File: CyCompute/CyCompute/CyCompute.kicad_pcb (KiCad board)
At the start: 2 copper layers, 100 x 140 mm, 29 parts, among them J1 RJ45, J10 RJ11, J11 RJ11, J12 RJ11, J13 RJ11, J14 RJ45, J15 RJ11, J16 USB_A, J17 USB_A, J18 Conn_01x04_Female, J2 RJ45, J3 RJ45, J4 RJ45, J5 RJ45, J6 CAM0, J7 CAM1, J8 Pi Std header, J9 RJ11, U1 TCA9548APWR, U2 LAN9514, U3 P82B715DR, U4 IP4234CZ6, U5 IP4234CZ6, U6 PAM2306AYPKE, U7 SP2526A-2EN-L

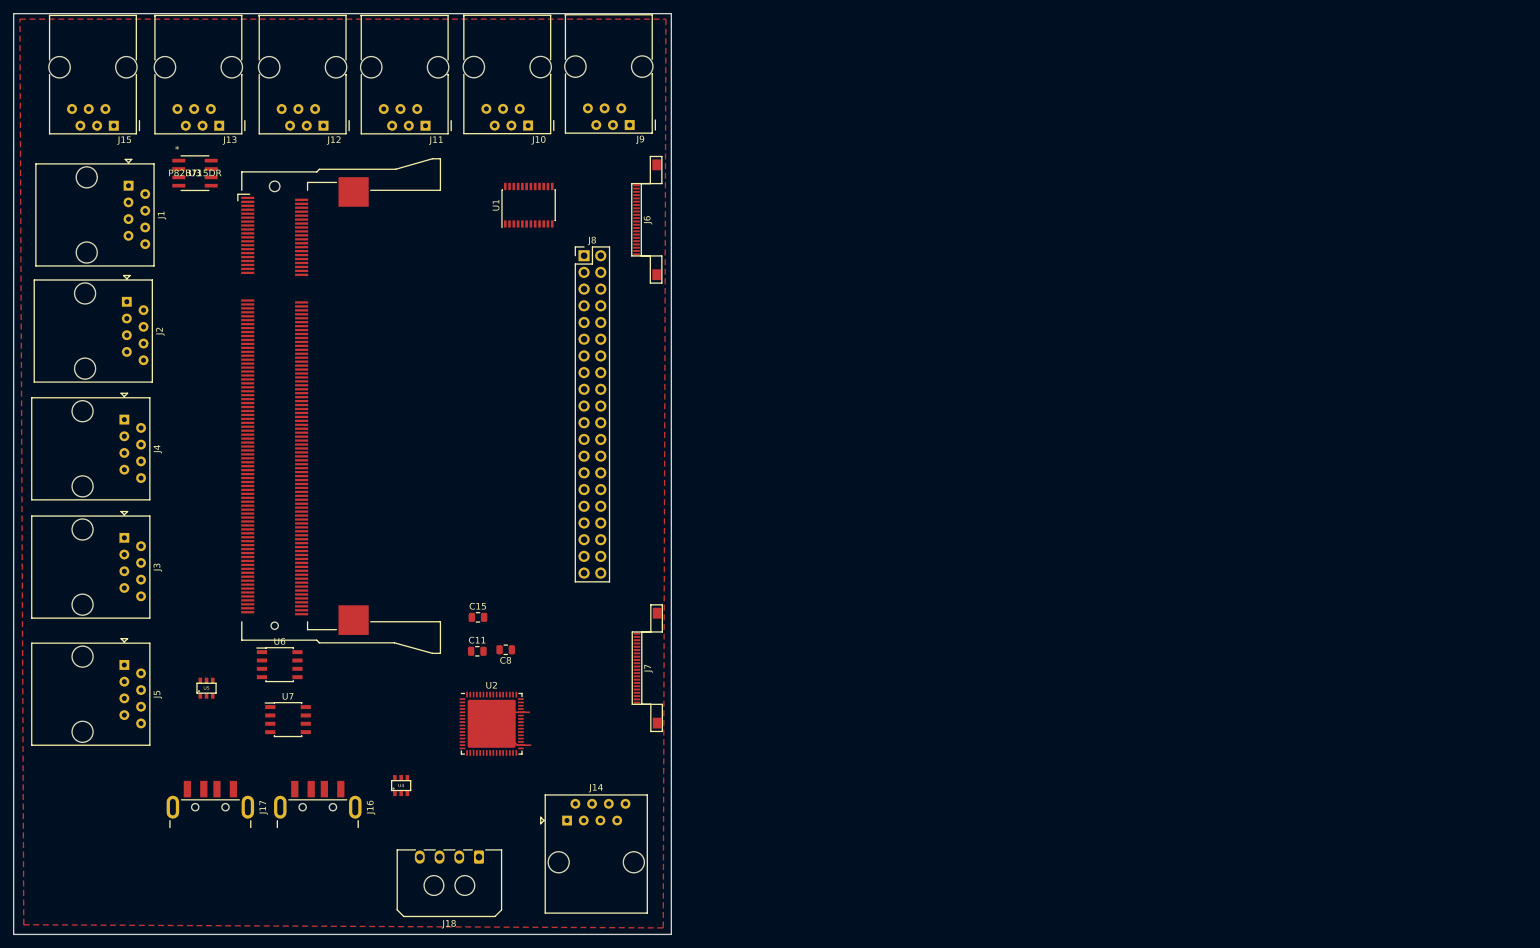
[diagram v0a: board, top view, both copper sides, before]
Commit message: Getting up to date
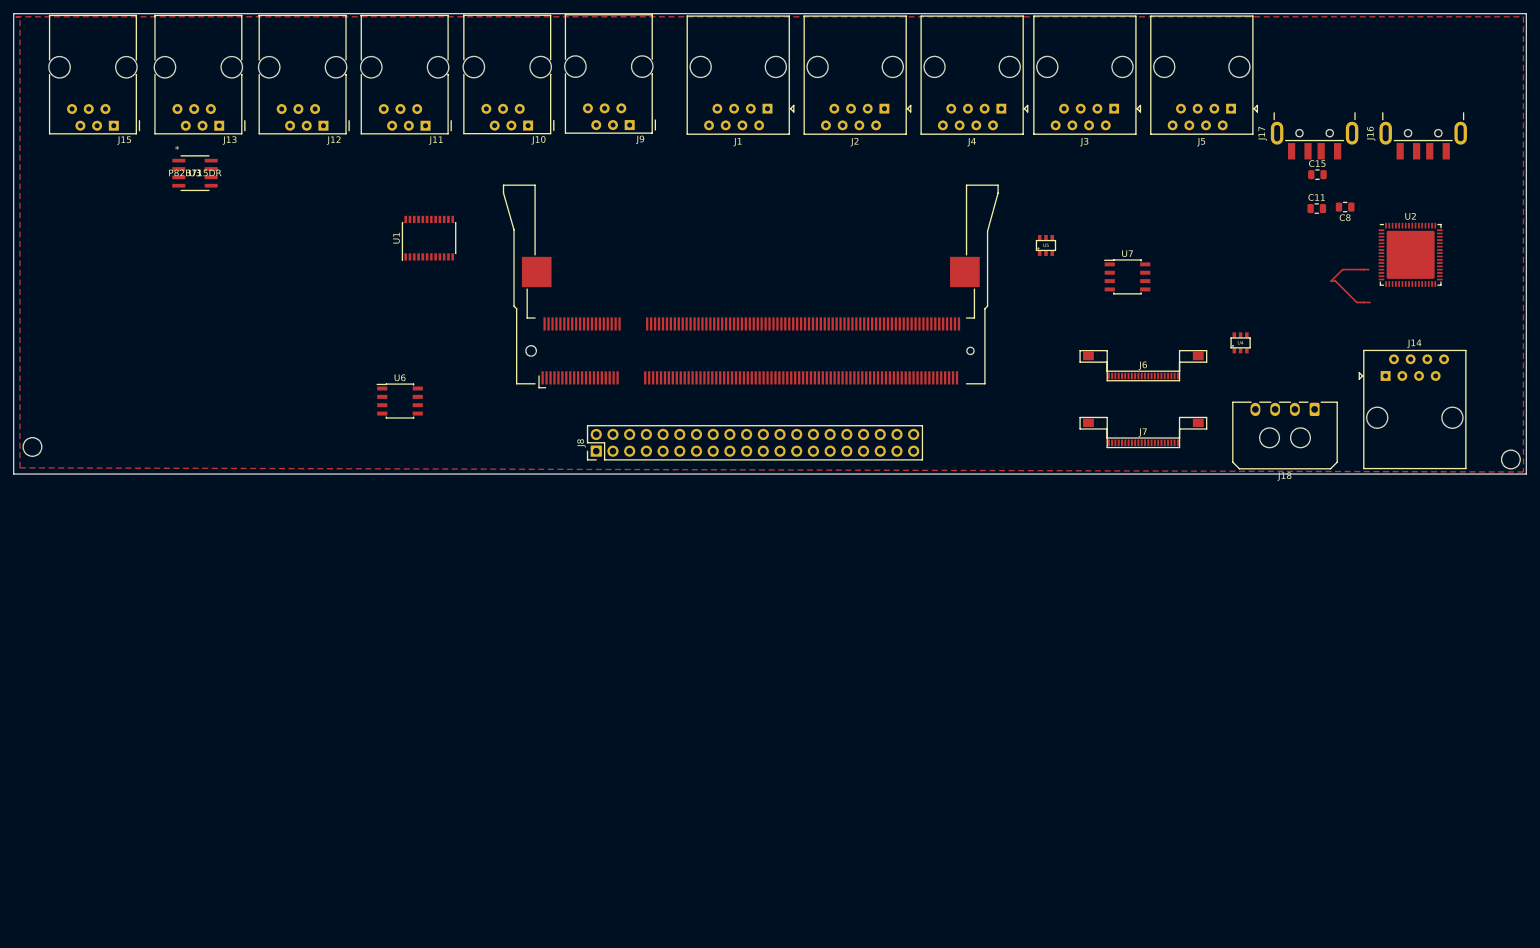
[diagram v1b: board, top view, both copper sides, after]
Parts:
- moved J16 204.4 mm to (234.3, 41.3), turned to 90 degrees
- moved J17 204.2 mm to (217.8, 41.3), turned to 90 degrees
- moved J5 188.3 mm to (205.1, 44.5), turned to 180 degrees
- moved J3 164.0 mm to (187.3, 44.5), turned to 180 degrees
- moved U2 156.9 mm to (232.4, 66.7)
- moved C8 144.3 mm to (222.5, 59.4)
- moved U5 144.3 mm to (177.0, 65.3)
- moved C11 144.3 mm to (218.1, 59.6)
- moved C15 144.3 mm to (218.2, 54.5)
- moved U4 144.3 mm to (206.6, 80.1)
- moved U7 144.3 mm to (189.4, 70.0)
- moved J18 144.1 mm to (217.8, 90.2)
- moved J14 141.6 mm to (228.6, 85.1)
- moved J4 141.5 mm to (170.2, 44.5), turned to 180 degrees
- moved J2 118.9 mm to (152.4, 44.5), turned to 180 degrees
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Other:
- board size 100 x 140 mm -> 230 x 70 mm
